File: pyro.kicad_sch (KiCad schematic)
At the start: 34 parts, among them J15 DB141R-2.54-8P-GN, Q1 MJD44H11T4G, Q10 PJM09P30DF, Q11 PJM09P30DF, Q12 PJM09P30DF, Q13 PJM09P30DF, Q5 NMOS, Q6 NMOS, Q7 NMOS, Q8 NMOS, Q9 NMOS, U6 LT3092xST

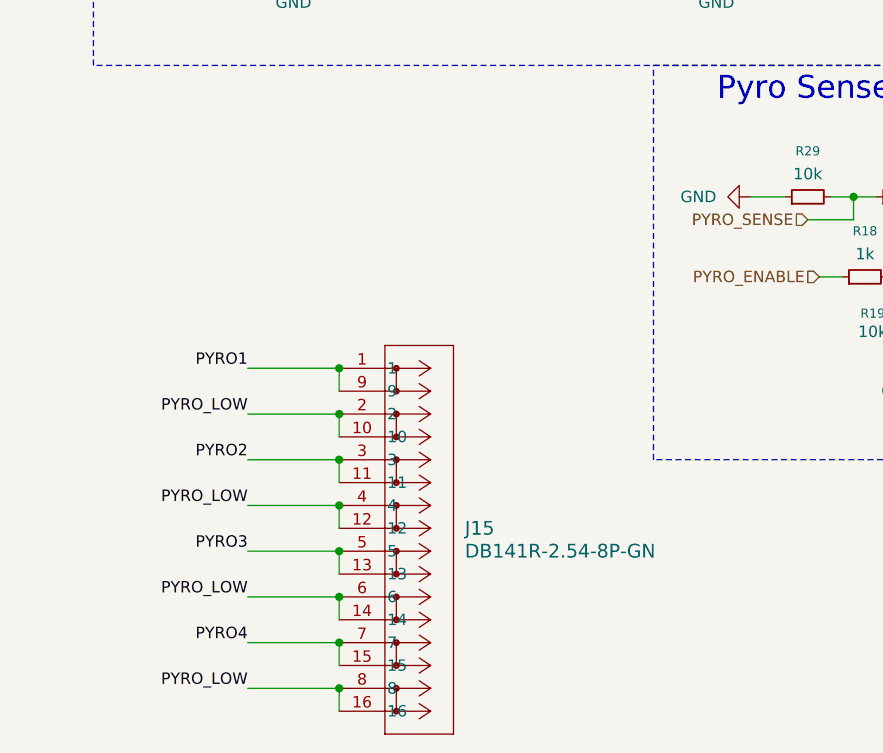
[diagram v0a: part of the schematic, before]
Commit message: led e buzzer
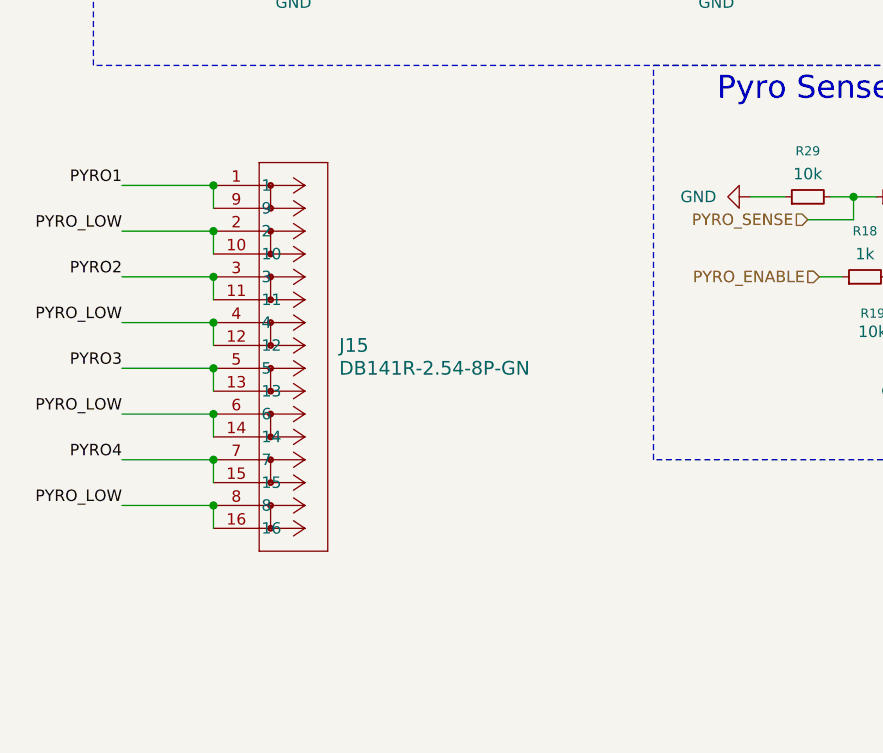
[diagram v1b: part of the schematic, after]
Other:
- moved on the sheet: J15
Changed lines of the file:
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@@
 	)
 	(junction
-		(at 78.74 173.99)
+		(at 64.77 153.67)
 		(diameter 0)
 		(color 0 0 0 0)
@@
 	)
 	(junction
-		(at 78.74 168.91)
+		(at 64.77 148.59)
 		(diameter 0)
 		(color 0 0 0 0)
@@
 	)
 	(junction
-		(at 78.74 179.07)
+		(at 64.77 158.75)
 		(diameter 0)
 		(color 0 0 0 0)
 	)
 	(junction
-		(at 78.74 158.75)
+		(at 64.77 138.43)
 		(diameter 0)
 		(color 0 0 0 0)
@@
 	)
 	(junction
-		(at 78.74 184.15)
+		(at 64.77 163.83)
 		(diameter 0)
 		(color 0 0 0 0)
 	)
 	(junction
-		(at 78.74 153.67)
+		(at 64.77 133.35)
 		(diameter 0)
 		(color 0 0 0 0)
@@
 	)
 	(junction
-		(at 78.74 148.59)
+		(at 64.77 128.27)
 		(diameter 0)
 		(color 0 0 0 0)
 	)
 	(junction
-		(at 78.74 163.83)
+		(at 64.77 143.51)
 		(diameter 0)
 		(color 0 0 0 0)
@@
 	(wire
 		(pts
-			(xy 78.74 173.99) (xy 78.74 176.53)
-		)
-		(stroke
-			(width 0)
-			(type default)
-		)
-	)
-	(wire
-		(pts
-			(xy 78.74 163.83) (xy 78.74 166.37)
+			(xy 64.77 153.67) (xy 64.77 156.21)
+		)
+		(stroke
+			(width 0)
+			(type default)
+		)
+	)
+	(wire
+		(pts
+			(xy 64.77 143.51) (xy 64.77 146.05)
 		)
 		(stroke
@@
 	(wire
 		(pts
-			(xy 78.74 148.59) (xy 78.74 151.13)
+			(xy 64.77 128.27) (xy 64.77 130.81)
 		)
 		(stroke
@@
 	(wire
 		(pts
-			(xy 78.74 184.15) (xy 78.74 186.69)
+			(xy 64.77 163.83) (xy 64.77 166.37)
 		)
 		(stroke
@@
 	(wire
 		(pts
-			(xy 68.58 153.67) (xy 78.74 153.67)
+			(xy 54.61 133.35) (xy 64.77 133.35)
 		)
 		(stroke
@@
 	(wire
 		(pts
-			(xy 68.58 173.99) (xy 78.74 173.99)
+			(xy 54.61 153.67) (xy 64.77 153.67)
 		)
 		(stroke
@@
 	(wire
 		(pts
-			(xy 78.74 153.67) (xy 78.74 156.21)
-		)
-		(stroke
-			(width 0)
-			(type default)
-		)
-	)
-	(wire
-		(pts
-			(xy 68.58 168.91) (xy 78.74 168.91)
+			(xy 64.77 133.35) (xy 64.77 135.89)
+		)
+		(stroke
+			(width 0)
+			(type default)
+		)
+	)
+	(wire
+		(pts
+			(xy 54.61 148.59) (xy 64.77 148.59)
 		)
 		(stroke
@@
 	(wire
 		(pts
-			(xy 78.74 158.75) (xy 78.74 161.29)
+			(xy 64.77 138.43) (xy 64.77 140.97)
 		)
 		(stroke
@@
 	(wire
 		(pts
-			(xy 68.58 158.75) (xy 78.74 158.75)
-		)
-		(stroke
-			(width 0)
-			(type default)
-		)
-	)
-	(wire
-		(pts
-			(xy 68.58 163.83) (xy 78.74 163.83)
+			(xy 54.61 138.43) (xy 64.77 138.43)
+		)
+		(stroke
+			(width 0)
+			(type default)
+		)
+	)
+	(wire
+		(pts
+			(xy 54.61 143.51) (xy 64.77 143.51)
 		)
 		(stroke
@@
 	(wire
 		(pts
-			(xy 68.58 184.15) (xy 78.74 184.15)
+			(xy 54.61 163.83) (xy 64.77 163.83)
 		)
 		(stroke
@@
 	(wire
 		(pts
-			(xy 68.58 179.07) (xy 78.74 179.07)
+			(xy 54.61 158.75) (xy 64.77 158.75)
 		)
 		(stroke
@@
 	(wire
 		(pts
-			(xy 78.74 179.07) (xy 78.74 181.61)
+			(xy 64.77 158.75) (xy 64.77 161.29)
 		)
 		(stroke
@@
 	(wire
 		(pts
-			(xy 68.58 148.59) (xy 78.74 148.59)
-		)
-		(stroke
-			(width 0)
-			(type default)
-		)
-	)
-	(wire
-		(pts
-			(xy 78.74 168.91) (xy 78.74 171.45)
+			(xy 54.61 128.27) (xy 64.77 128.27)
+		)
+		(stroke
+			(width 0)
+			(type default)
+		)
+	)
+	(wire
+		(pts
+			(xy 64.77 148.59) (xy 64.77 151.13)
 		)
 		(stroke
@@
 	)
 	(label "PYRO_LOW"
-		(at 68.58 173.99 180)
+		(at 54.61 153.67 180)
 		(effects
 			(font
@@
 	)
 	(label "PYRO_LOW"
-		(at 68.58 163.83 180)
+		(at 54.61 143.51 180)
 		(effects
 			(font
@@
 	)
 	(label "PYRO2"
-		(at 68.58 158.75 180)
+		(at 54.61 138.43 180)
 		(effects
 			(font
@@
 	)
 	(label "PYRO3"
-		(at 68.58 168.91 180)
+		(at 54.61 148.59 180)
 		(effects
 			(font
@@
 	)
 	(label "PYRO4"
-		(at 68.58 179.07 180)
+		(at 54.61 158.75 180)
 		(effects
 			(font
@@
 	)
 	(label "PYRO_LOW"
-		(at 68.58 184.15 180)
+		(at 54.61 163.83 180)
 		(effects
 			(font
@@
 	)
 	(label "PYRO_LOW"
-		(at 68.58 153.67 180)
+		(at 54.61 133.35 180)
 		(effects
 			(font
@@
 	)
 	(label "PYRO1"
-		(at 68.58 148.59 180)
+		(at 54.61 128.27 180)
 		(effects
 			(font
@@
 	(symbol
 		(lib_id "2025-09-27_12-32-40:DB141R-2.54-8P-GN")
-		(at 78.74 148.59 0)
+		(at 64.77 128.27 0)
 		(unit 1)
 		(exclude_from_sim no)
@@
 		(fields_autoplaced yes)
 		(property "Reference" "J15"
-			(at 92.71 166.3699 0)
+			(at 78.74 146.0499 0)
 			(effects
 				(font
@@
 		)
 		(property "Value" "DB141R-2.54-8P-GN"
-			(at 92.71 168.9099 0)
+			(at 78.74 148.5899 0)
 			(effects
 				(font
@@
 		)
 		(property "Footprint" "DB141R-2-54-8:CONN16_DB141R_DIO"
-			(at 78.74 148.59 0)
+			(at 64.77 128.27 0)
 			(effects
 				(font
@@
 		)
 		(property "Datasheet" "DB141R-2.54-8P-GN"
-			(at 78.74 148.59 0)
+			(at 64.77 128.27 0)
 			(effects
 				(font
@@
 		)
 		(property "Description" ""
-			(at 78.74 148.59 0)
-			(effects
-				(font
+			(at 64.77 128.27 0)
+			(effects
+				(font
